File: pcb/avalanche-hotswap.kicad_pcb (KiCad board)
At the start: 2 copper layers, 179.4 x 124.3 mm, 138 parts, among them J1 TRRS, J2 OLED, P1 i2c_pin, P2 i2c_pin, P3 battery+, P4 battery-, SW0 SW_Push, SW1 SW_Push, SW10 SW_Push, SW11 SW_Push, SW12 SW_Push, SW13 SW_Push, SW14 SW_Push, SW15 SW_Push, SW16 SW_Push, SW17 SW_Push, SW18 SW_Push, SW19 SW_Push, SW2 SW_Push, SW20 SW_Push, SW21 SW_Push, SW22 SW_Push, SW23 SW_Push, SW24 SW_Push, SW25 SW_Push, SW26 SW_Push, SW27 SW_Push, SW28 SW_Push, SW29 SW_Push, SW3 SW_Push, SW30 SW_Push, SW31 SW_Push, SW32 SW_Push, SW33 SW_DPDT_x2, SW34 SW_DPDT_x2, SW4 SW_Push, SW5 SW_Push, SW6 SW_Push, SW7 SW_Push, SW8 SW_Push, SW9 SW_Push, U1 ProMicro

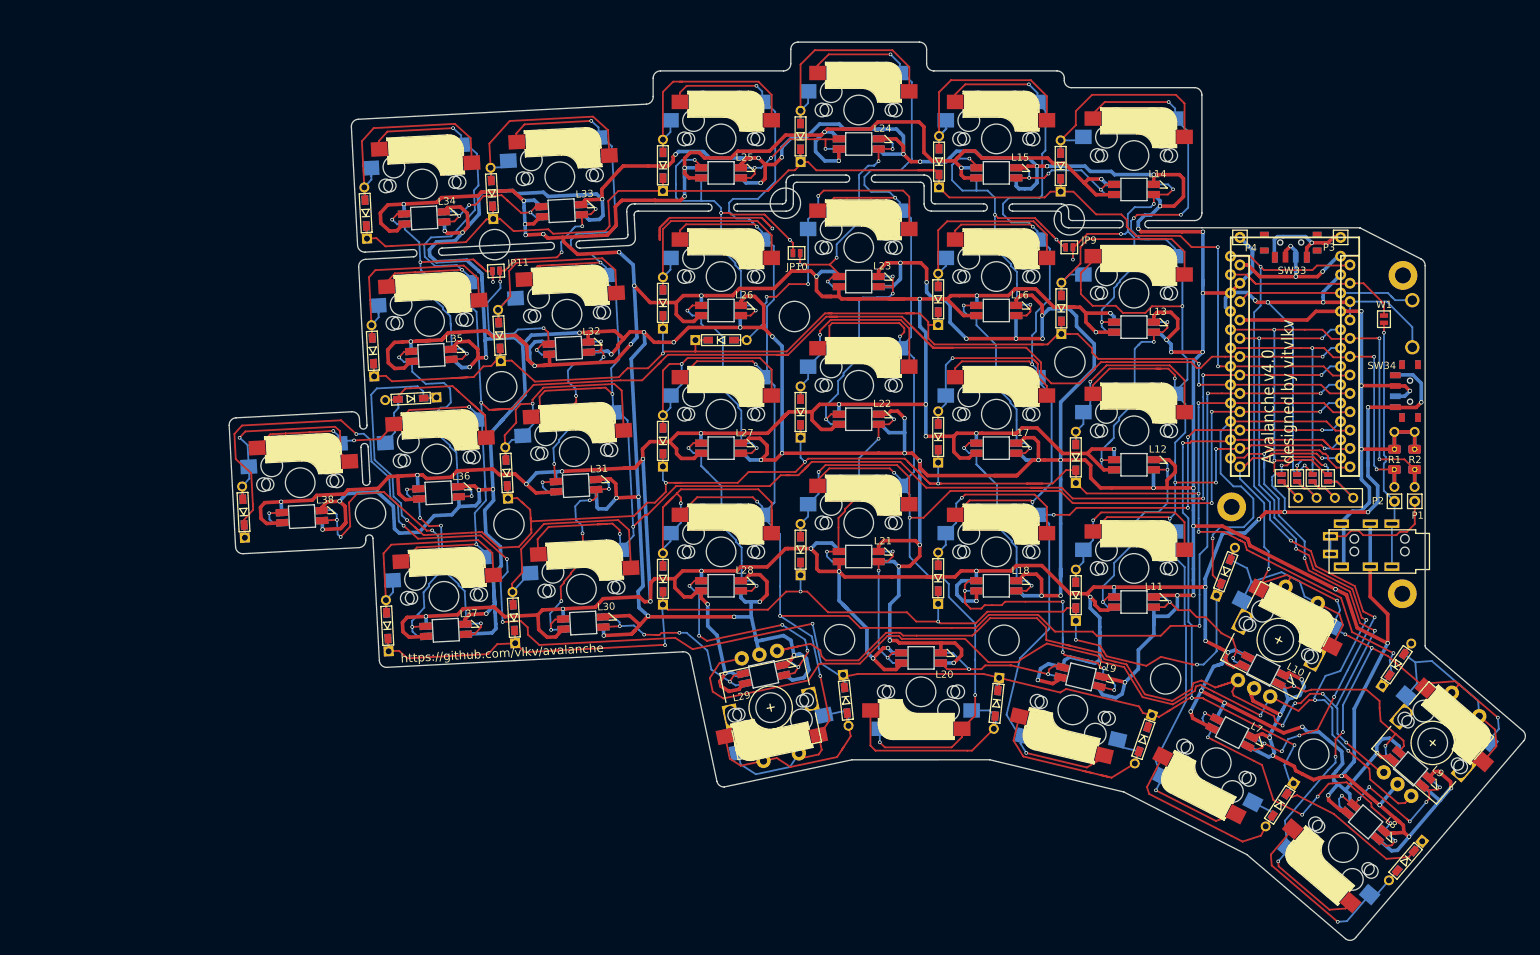
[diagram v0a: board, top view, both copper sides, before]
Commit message: WIP
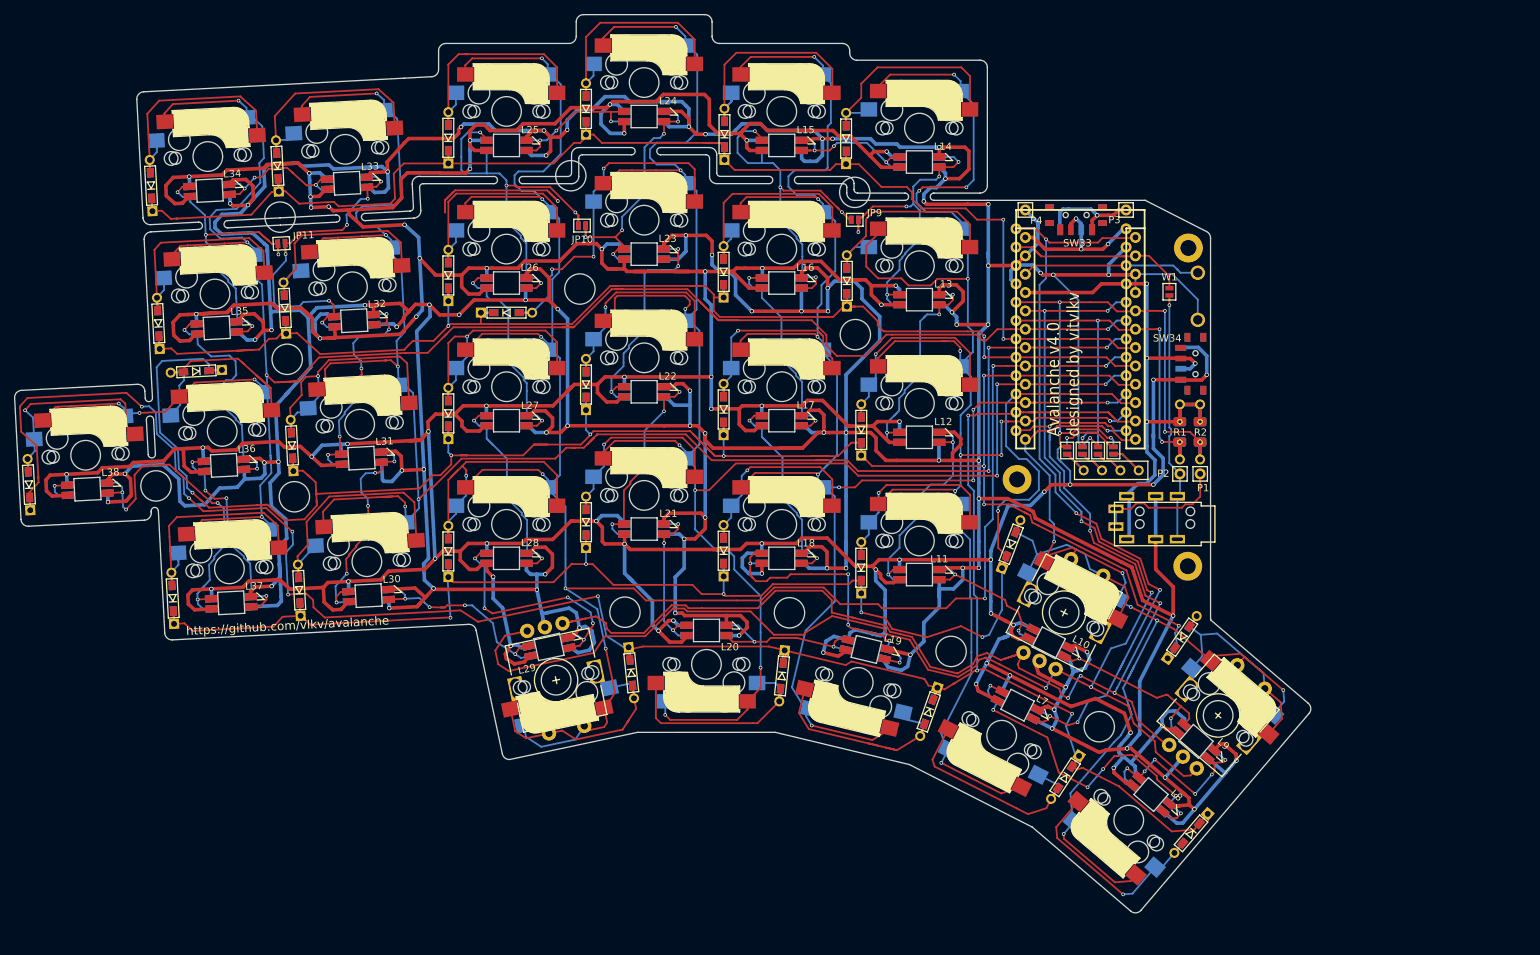
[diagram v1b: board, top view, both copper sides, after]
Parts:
- moved SW25 29.9 mm to (151.6, 98.8)
- moved D23 29.9 mm to (105.4, 96.2)
- moved D13 29.9 mm to (51.5, 75.3)
- moved JP7 29.9 mm to (176.3, 86.2)
- moved L26 29.9 mm to (94.4, 63.1)
- moved SW27 29.9 mm to (36.2, 86.9)
- moved L35 29.9 mm to (54.3, 69.3)
- moved SW24 29.9 mm to (132.5, 96.5)
- moved L38 29.9 mm to (36.4, 91.6)
- moved D17 29.9 mm to (124.5, 80.6)
- moved D12 29.9 mm to (141.5, 62.8)
- moved R2 29.9 mm to (190.4, 83.7)
- moved L33 29.9 mm to (72.4, 49.2)
- moved SW18 29.9 mm to (151.6, 79.7)
- moved L34 29.9 mm to (53.3, 50.2)
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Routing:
- net col6: track 133.3 -> 136.8 mm, vias 9 -> 7
- net VCC: track 981.3 -> 977.9 mm
- net Net-(L10-Pad4): track 30.6 -> 28.5 mm
- net LED: track 106.4 -> 107.7 mm, vias 7 -> 5
- net encA: track 180.3 -> 179.5 mm, vias 7 -> 6
- net encB: track 202.0 -> 201.3 mm, vias 7 -> 6
- net row4: track 307.3 -> 306.7 mm
- net GND: track 1147.0 -> 1147.1 mm, vias 78 -> 77

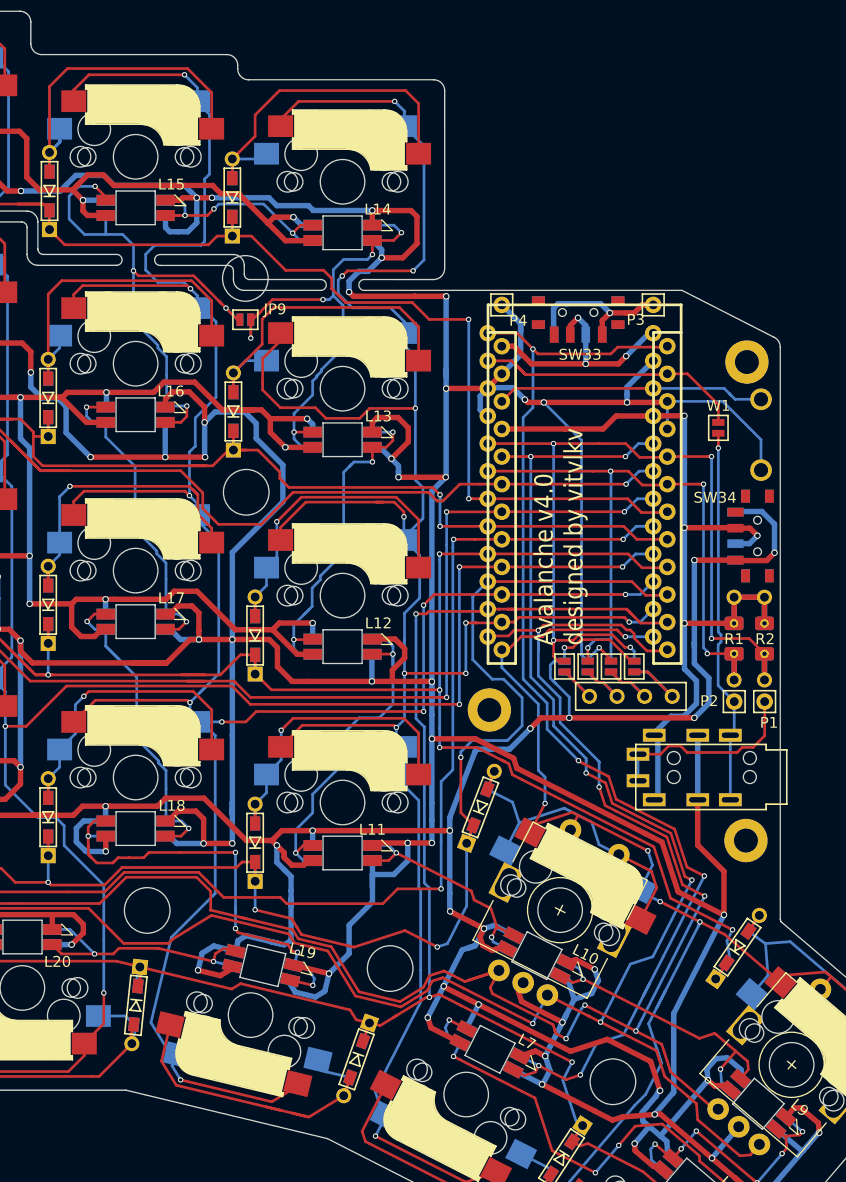
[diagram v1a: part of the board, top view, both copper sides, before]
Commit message: Changing stagger
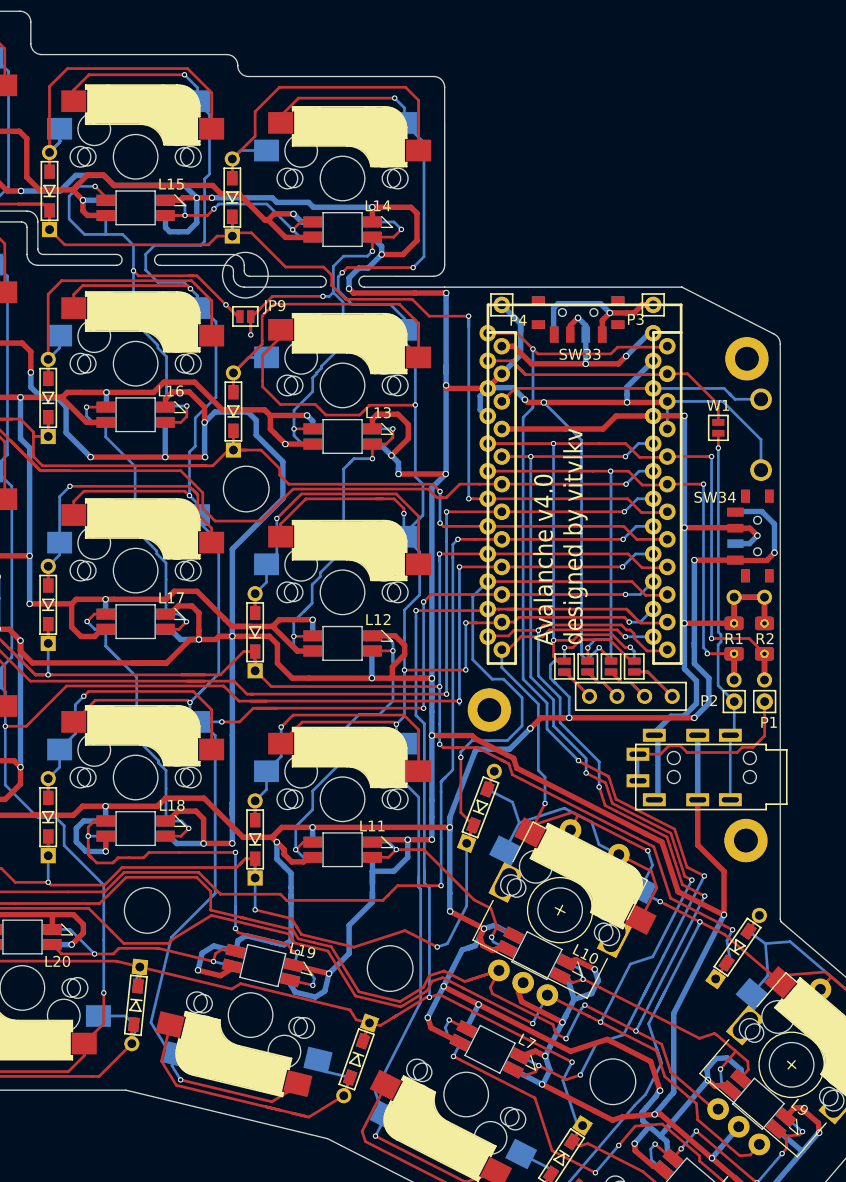
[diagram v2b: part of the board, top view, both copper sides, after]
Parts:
- moved L11 0.30 mm to (151.6, 103.1)
- moved L13 0.30 mm to (151.6, 65.1)
- moved HM1 0.30 mm to (188.8, 57.9)
- moved L14 0.30 mm to (151.6, 46.0)
- moved SW12 0.30 mm to (151.6, 60.4)
- moved D18 0.30 mm to (143.5, 83.1)
- moved D25 0.30 mm to (143.5, 102.2)
- moved HM10 0.30 mm to (142.7, 69.9)
- moved HM2 0.30 mm to (142.6, 50.2)
- moved JP9 0.30 mm to (142.6, 54.0)
- moved L12 0.30 mm to (151.6, 84.1)
- moved SW18 0.30 mm to (151.6, 79.4)
- moved SW25 0.30 mm to (151.6, 98.5)
- moved SW6 0.30 mm to (151.6, 41.3)
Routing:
- net col4: track 228.7 -> 231.1 mm
- net Net-(D6-Pad2): track 32.3 -> 34.0 mm
- net col3: track 263.0 -> 264.4 mm
- net row4: track 306.7 -> 308.0 mm
- net GND: track 1147.1 -> 1148.3 mm
- net row0: track 192.6 -> 193.6 mm
- net VCC: track 977.9 -> 977.0 mm
- net row3: track 217.8 -> 218.5 mm
- net col5: track 220.7 -> 221.3 mm
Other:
- outline, holes or cut-outs redrawn
